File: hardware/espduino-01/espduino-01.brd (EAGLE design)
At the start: 15.5 x 34.9 mm, 21 parts, among them U1 FT231XS

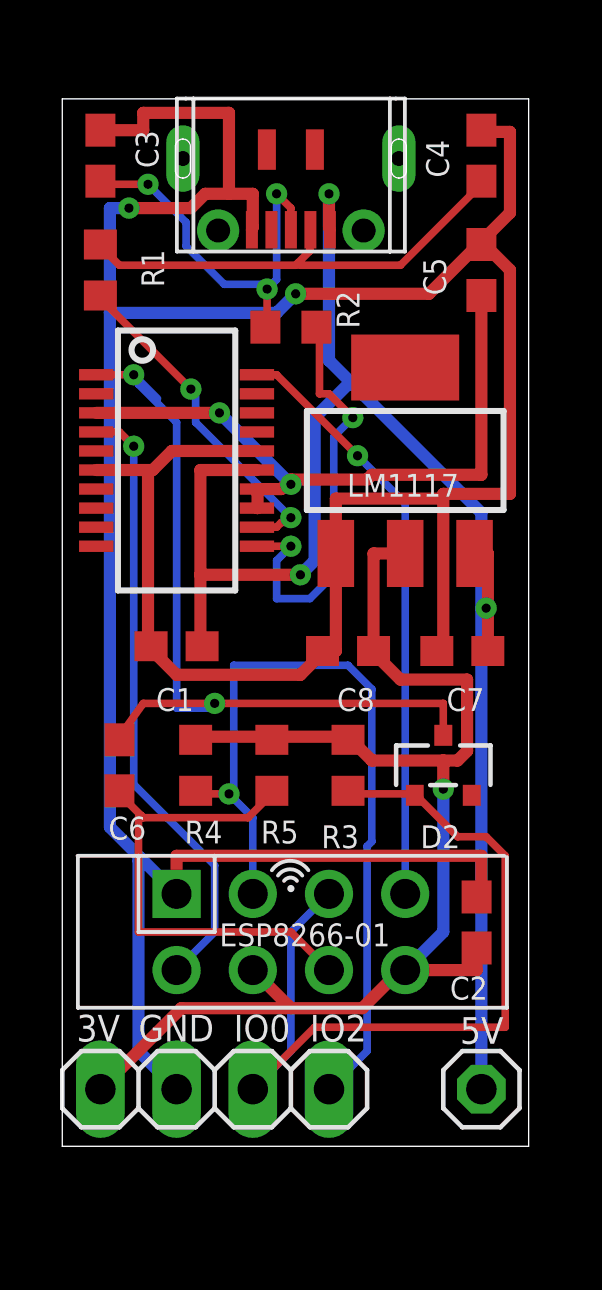
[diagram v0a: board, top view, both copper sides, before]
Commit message: Rev 2 of espduino-m2
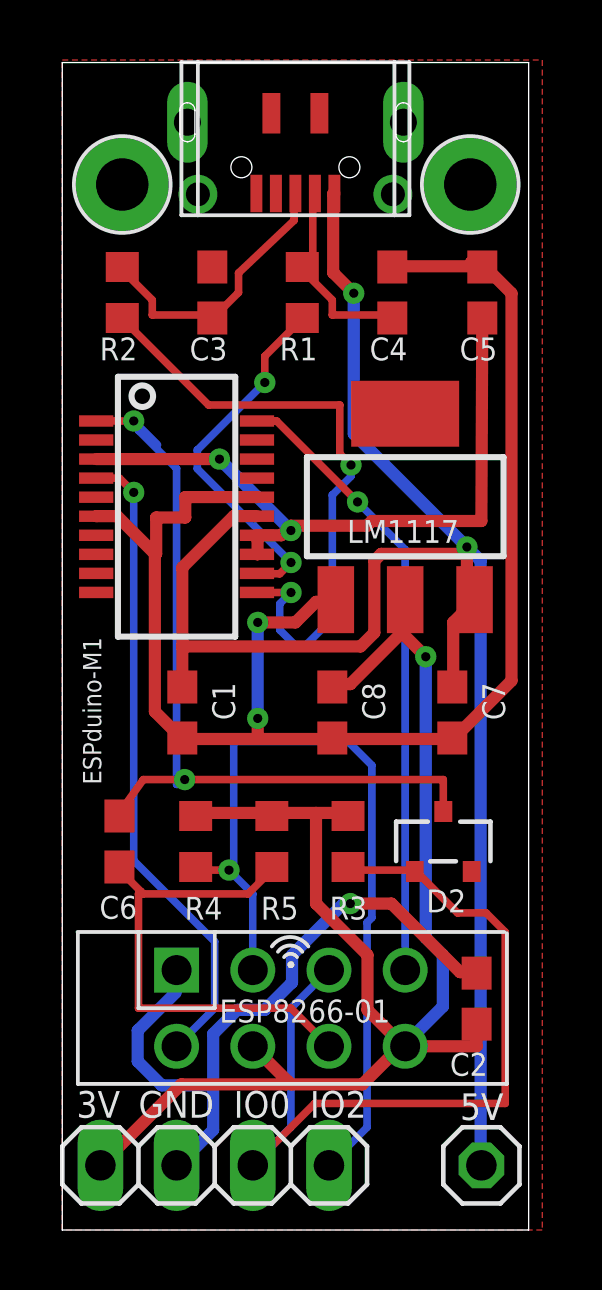
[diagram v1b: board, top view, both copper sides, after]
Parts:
- added U$2, U$3: MOUNTING-HOLEM1.6, jumper-parts:M1_6MOUNTING_HOLE
- U$1: device jumper-parts:JUMPER-LOGO-SMALL -> jumper-parts:JUMPER-LOGO-X-SMALL
- moved R1 6.77 mm to (8.00, 31.0)
- moved C3 5.89 mm to (5.00, 31.0)
- moved R2 5.74 mm to (2.00, 31.0), turned to 90 degrees
- moved C4 5.44 mm to (11.0, 31.0)
- moved U$1 3.49 mm to (9.50, 24.5)
- moved C2 2.54 mm to (13.8, 7.46)
- moved C6 2.54 mm to (1.91, 12.7)
- moved D2 2.54 mm to (12.7, 12.7)
- moved R3 2.54 mm to (9.53, 12.7)
- moved R4 2.54 mm to (4.45, 12.7)
- moved R5 2.54 mm to (6.99, 12.7)
- moved 5V 2.54 mm to (14.0, 1.91)
- moved ESP8266 2.54 mm to (5.08, 1.91)
- moved ESP8266-01 2.54 mm to (7.62, 7.14)
- moved C1 2.22 mm to (4.00, 17.0), turned to 270 degrees
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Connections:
- net GND: now also U$2.P$1, U$3.P$1
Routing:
- net GND: track 120.8 -> 74.0 mm, vias 2 -> 3
- net N$4: track 15.6 -> 7.62 mm
- net N$2: track 14.6 -> 20.9 mm
- net 3.3V: track 44.2 -> 50.2 mm
- net N$3: track 13.7 -> 9.84 mm, vias 3 -> 0
- net 5V: track 55.3 -> 59.1 mm, vias 3 -> 2
- net TXD: track 20.6 -> 21.6 mm
- net RXD: track 19.7 -> 20.7 mm
- net N$1: track 11.3 -> 12.2 mm
- net N$5: track 21.9 -> 22.7 mm
- added copper zone on layer 1, net GND
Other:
- board size 15.5 x 34.9 mm -> 15.5 x 38.9 mm
- board text added: "ESPduino-M1"
- board text removed: "ESPduino"
